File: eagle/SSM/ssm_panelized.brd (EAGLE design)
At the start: 73 x 100.3 mm, 69 parts, among them IC1 4051N, IC2 MCP604P, IC3 4051N, IC4 MCP604P, IC5 4051N, IC6 MCP604P

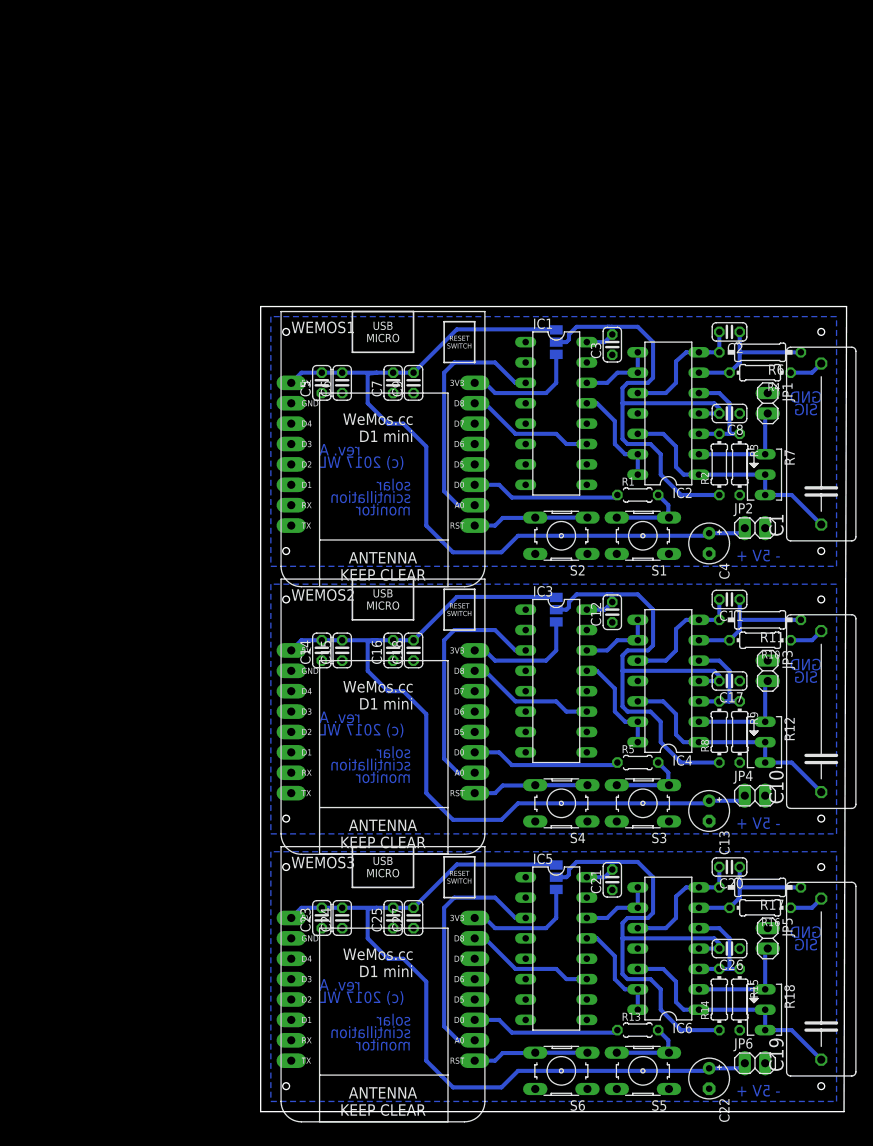
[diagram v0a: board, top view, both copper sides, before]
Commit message: move panels to 0,0
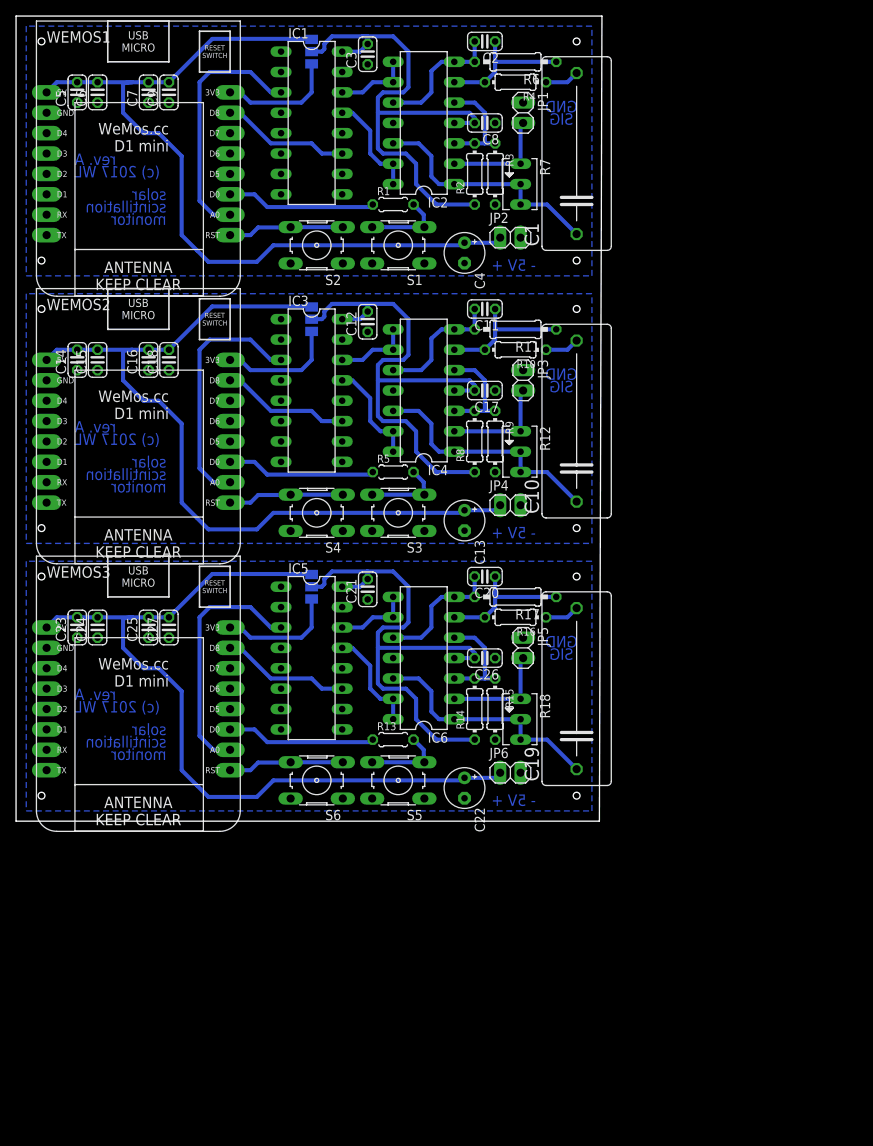
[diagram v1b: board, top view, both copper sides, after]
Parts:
- moved C11 47.3 mm to (58.4, 63.8)
- moved C5 47.3 mm to (7.62, 90.8)
- moved C6 47.3 mm to (10.2, 90.8)
- moved C7 47.3 mm to (16.5, 90.8)
- moved C8 47.3 mm to (58.4, 87.0)
- moved C9 47.3 mm to (19.1, 90.8)
- moved IC1 47.3 mm to (36.8, 87.0)
- moved IC2 47.3 mm to (50.8, 87.0)
- moved SJ1 47.3 mm to (36.8, 95.9)
- moved C1 47.3 mm to (69.8, 84.5)
- moved C10 47.3 mm to (69.8, 51.1)
- moved C13 47.3 mm to (55.9, 37.5)
- moved C14 47.3 mm to (7.62, 57.5)
- moved C15 47.3 mm to (10.2, 57.5)
- moved C16 47.3 mm to (16.5, 57.5)
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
